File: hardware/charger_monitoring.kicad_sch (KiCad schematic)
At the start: 18 parts, among them Q23 IPT015N10N5, Q24 IPT015N10N5, Q25 IRFR120NTRPBF, U2 BQ76200PW, U9 ACS724xLCTR-30AU

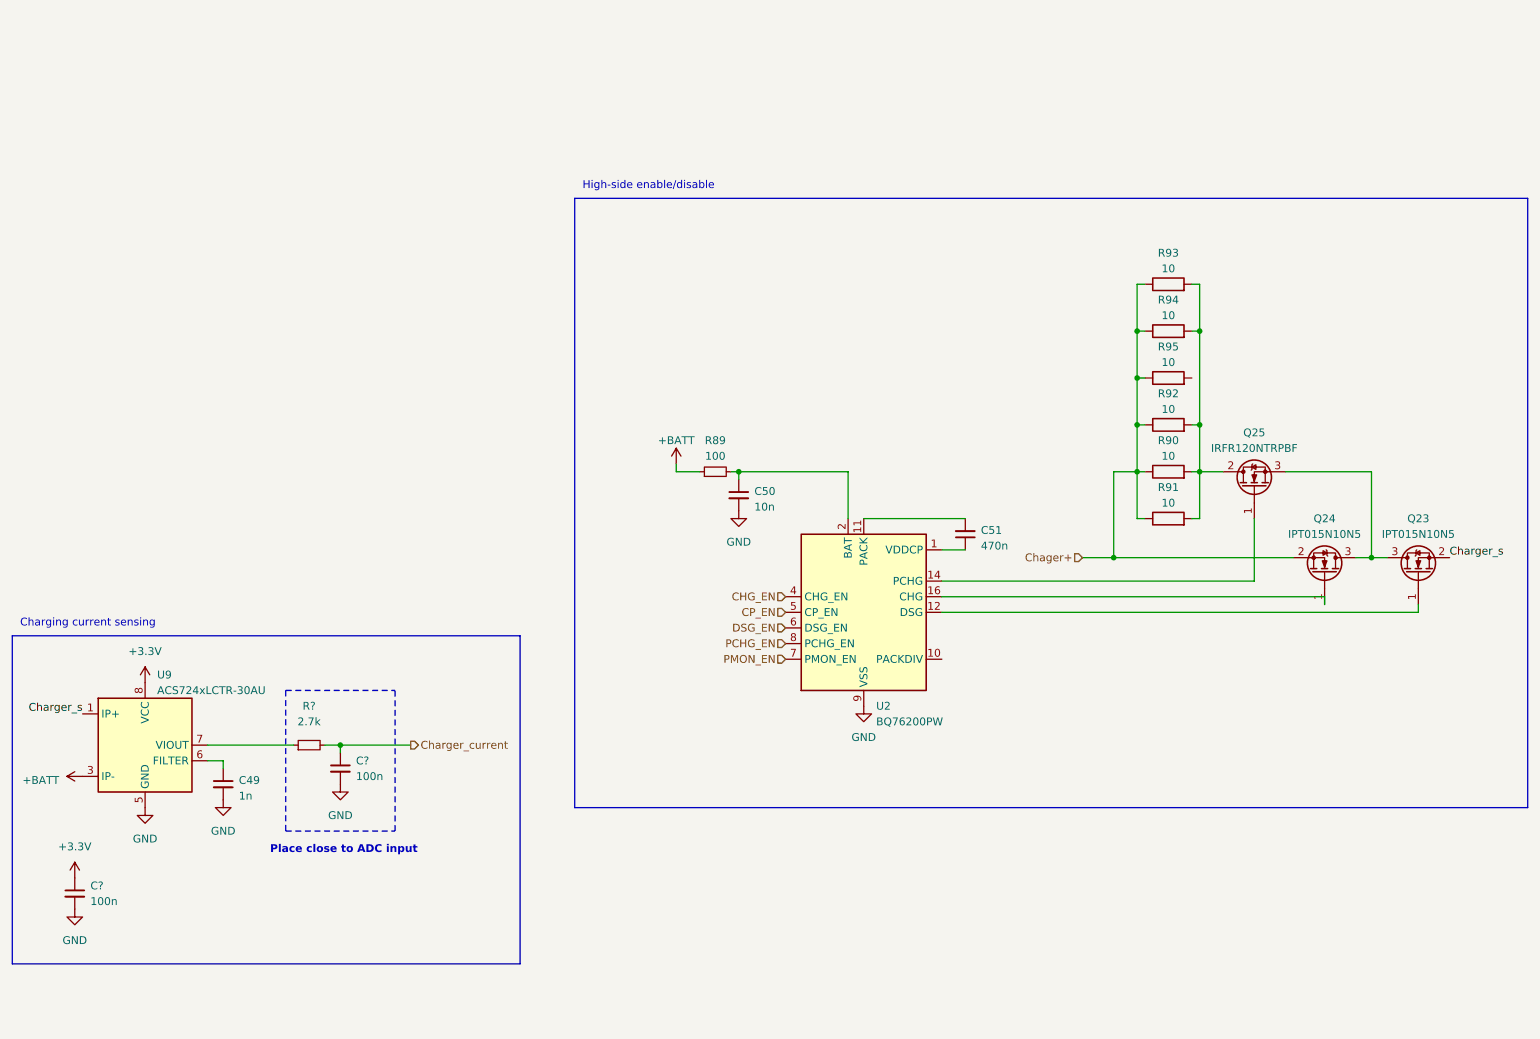
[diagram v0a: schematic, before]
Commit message: Charge monitor complete
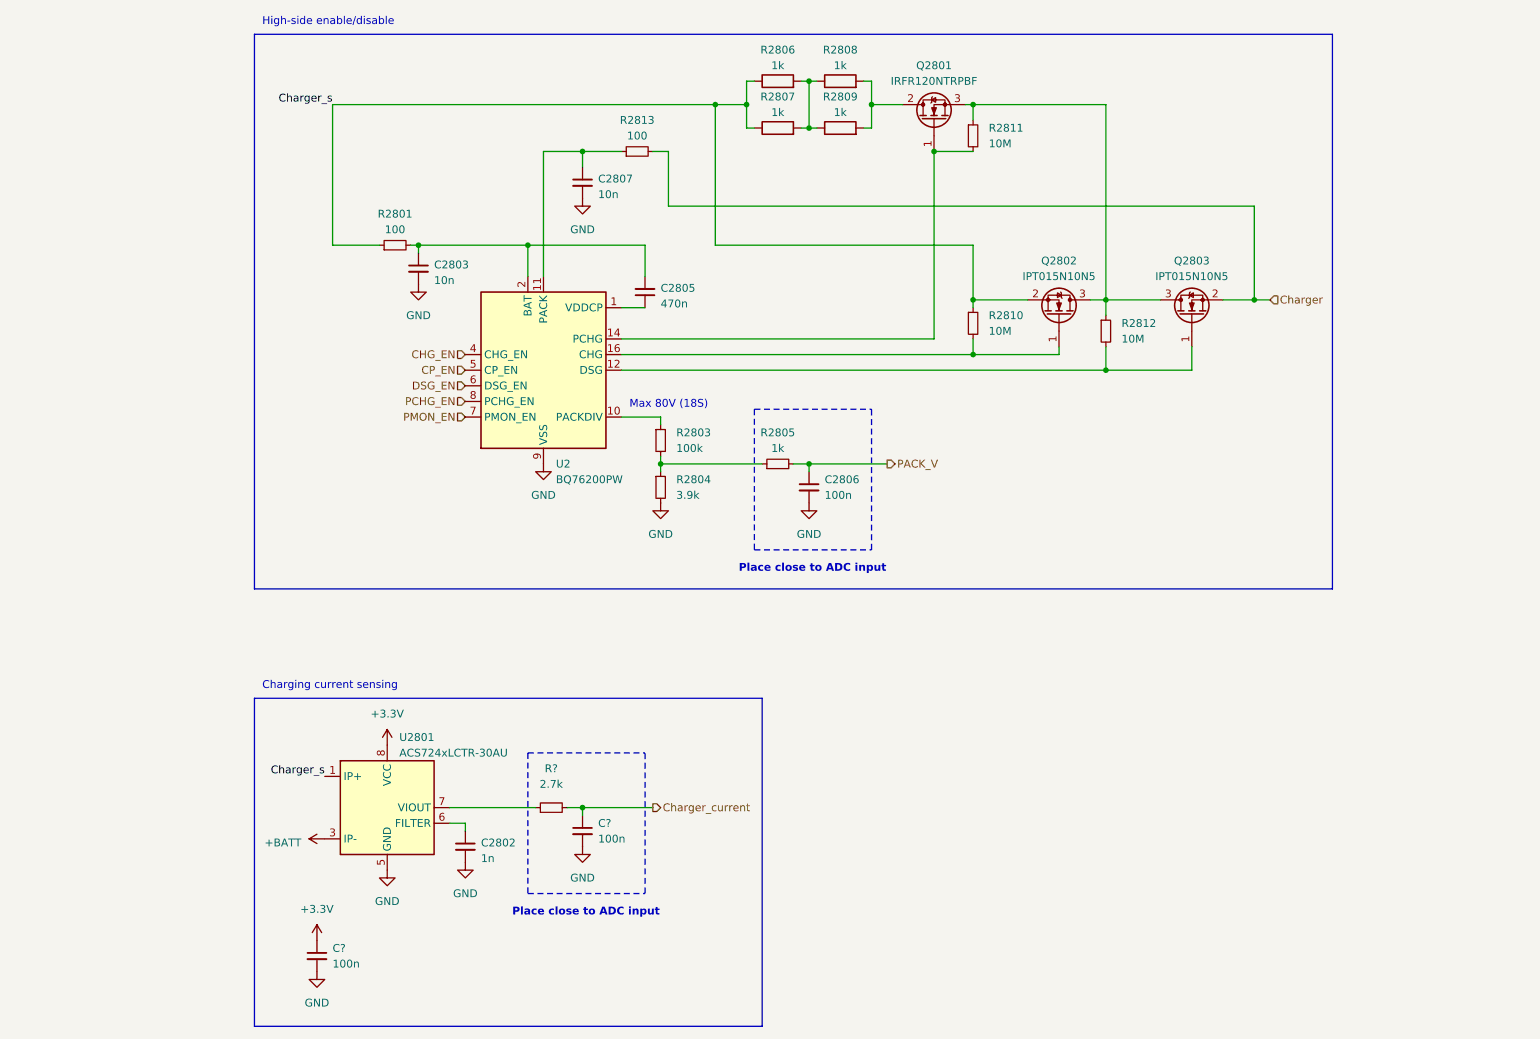
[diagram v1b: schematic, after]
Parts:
- removed R93, R94: 10, Resistor_SMD:R_2010_5025Metric, symbol Device:R
- added C2806: 100n, symbol Device:C_Small
- added C2807: 10n, symbol Device:C_Small
- added R2803: 100k, symbol Device:R_Small
- added R2804: 3.9k, symbol Device:R_Small
- added R2805: 1k, symbol Device:R_Small
- added R2810, R2811, R2812: 10M, symbol Device:R_Small
- added R2813: 100, symbol Device:R_Small
- R2806: renamed from R95; value 10 -> 1k; footprint Resistor_SMD:R_2010_5025Metric -> Resistor_SMD:R_2512_6332Metric
- R2807: renamed from R92; value 10 -> 1k; footprint Resistor_SMD:R_2010_5025Metric -> Resistor_SMD:R_2512_6332Metric
- R2808: renamed from R90; value 10 -> 1k; footprint Resistor_SMD:R_2010_5025Metric -> Resistor_SMD:R_2512_6332Metric
- R2809: renamed from R91; value 10 -> 1k; footprint Resistor_SMD:R_2010_5025Metric -> Resistor_SMD:R_2512_6332Metric
- renumbered C49 to C2802, C50 to C2803, C51 to C2805, Q25 to Q2801, Q24 to Q2802, Q23 to Q2803, R89 to R2801, U9 to U2801
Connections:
- net +BATT: no longer R2801.1
- net Charger_s: now also Q2802.2 (S), R2801.1, R2806.1, R2807.1, R2810.1; no longer Q2803.2 (S)
- net GND: now also C2806.2, C2807.2, R2804.2
- net at Q2801.2 (D), R2808.2, R2809.2: no longer R2807.2
- net at R2806.2: now also R2807.2, R2808.1, R2809.1
- net at Q2802.1 (G), U2.16 (CHG): now also R2810.2
- net at Q2801.3 (S), Q2802.3 (D), Q2803.3 (D): now also R2811.1, R2812.1
- net at C2803.1, R2801.2, U2.2 (BAT): now also C2805.2
- net at U2.10 (PACKDIV): now also R2803.1
- net at U2.11 (PACK): now also C2807.1, R2813.1; no longer C2805.2
- net at Q2803.1 (G), U2.12 (DSG): now also R2812.2
- net at Q2801.1 (G), U2.14 (PCHG): now also R2811.2
- removed net Chager+: Q2802.2 (S), R2806.1, R2807.1, R2808.1, R2809.1
- new net: R2803.2, R2804.1, R2805.1
- new net Charger: Q2803.2 (S), R2813.2
- new net PACK_V: C2806.1, R2805.2
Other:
- note added: "Max 80V (18S)"
- moved on the sheet: C2802, C2803, C2805, C?, Q2801, Q2802, Q2803, R2801, R2806, R2807, R2808, R2809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
